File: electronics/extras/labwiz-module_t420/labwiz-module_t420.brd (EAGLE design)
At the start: 66 x 31.5 mm, 48 parts, among them IC1 MCP3424, U1 MCP9800

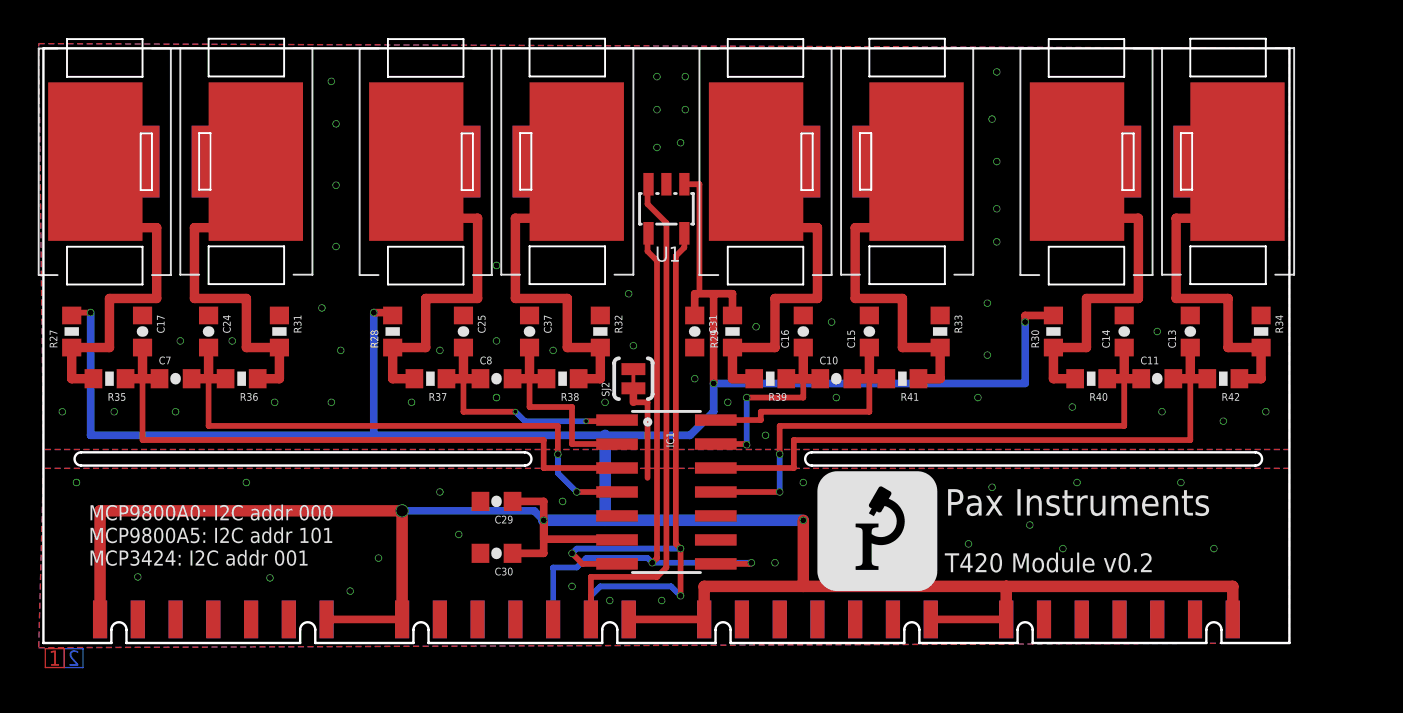
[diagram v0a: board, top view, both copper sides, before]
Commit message: Updated .gitignore. Comitting unknown schematic updates.
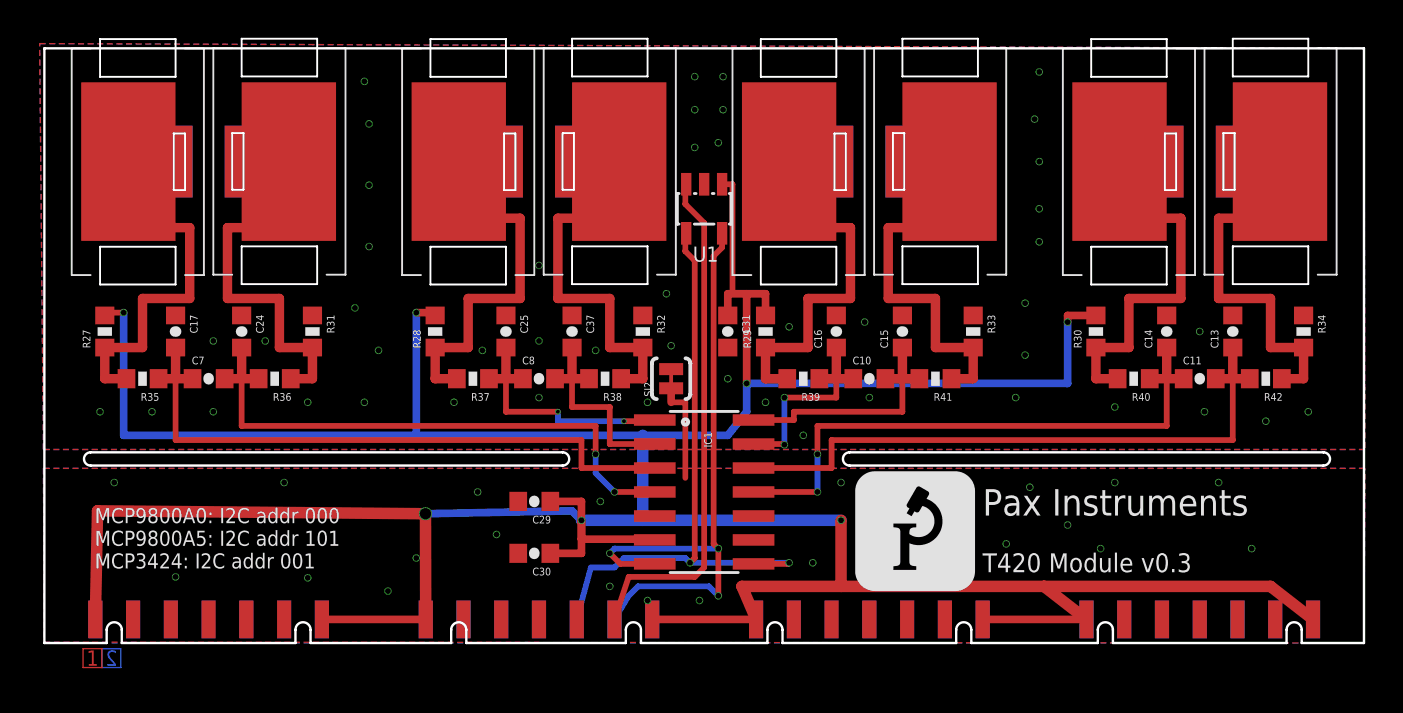
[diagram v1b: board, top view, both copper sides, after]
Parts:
- moved MODULE8 4.25 mm to (67.2, 1.00)
- moved MODULE7 2.75 mm to (49.8, 1.00)
- moved C11 2.25 mm to (61.2, 14.0)
- moved C13 2.25 mm to (63.0, 16.5)
- moved C14 2.25 mm to (59.5, 16.5)
- moved C25 2.25 mm to (24.5, 16.5)
- moved C37 2.25 mm to (28.0, 16.5)
- moved C8 2.25 mm to (26.2, 14.0)
- moved R28 2.25 mm to (20.8, 16.5)
- moved R30 2.25 mm to (55.8, 16.5)
- moved R32 2.25 mm to (31.8, 16.5)
- moved R34 2.25 mm to (66.8, 16.5)
- moved R37 2.25 mm to (22.8, 14.0)
- moved R38 2.25 mm to (29.8, 14.0)
- moved R40 2.25 mm to (57.8, 14.0)
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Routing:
- net 3.3V: track 201.2 -> 210.4 mm
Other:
- board size 66 x 31.5 mm -> 69.9 x 31.5 mm
- board text added: "T420 Module v0.3"
- board text removed: "T420 Module v0.2"
